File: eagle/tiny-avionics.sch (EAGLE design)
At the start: 62 parts, among them J1 USB-MICROB, J3 JST-PH-2-SMT-RA, U1 LP5907, U2 M25PX16, U3 LSM6DS3, U4 BQ21040, U5 LTC1998, U6 ATMEGA32U4-AU, X1 8MHz

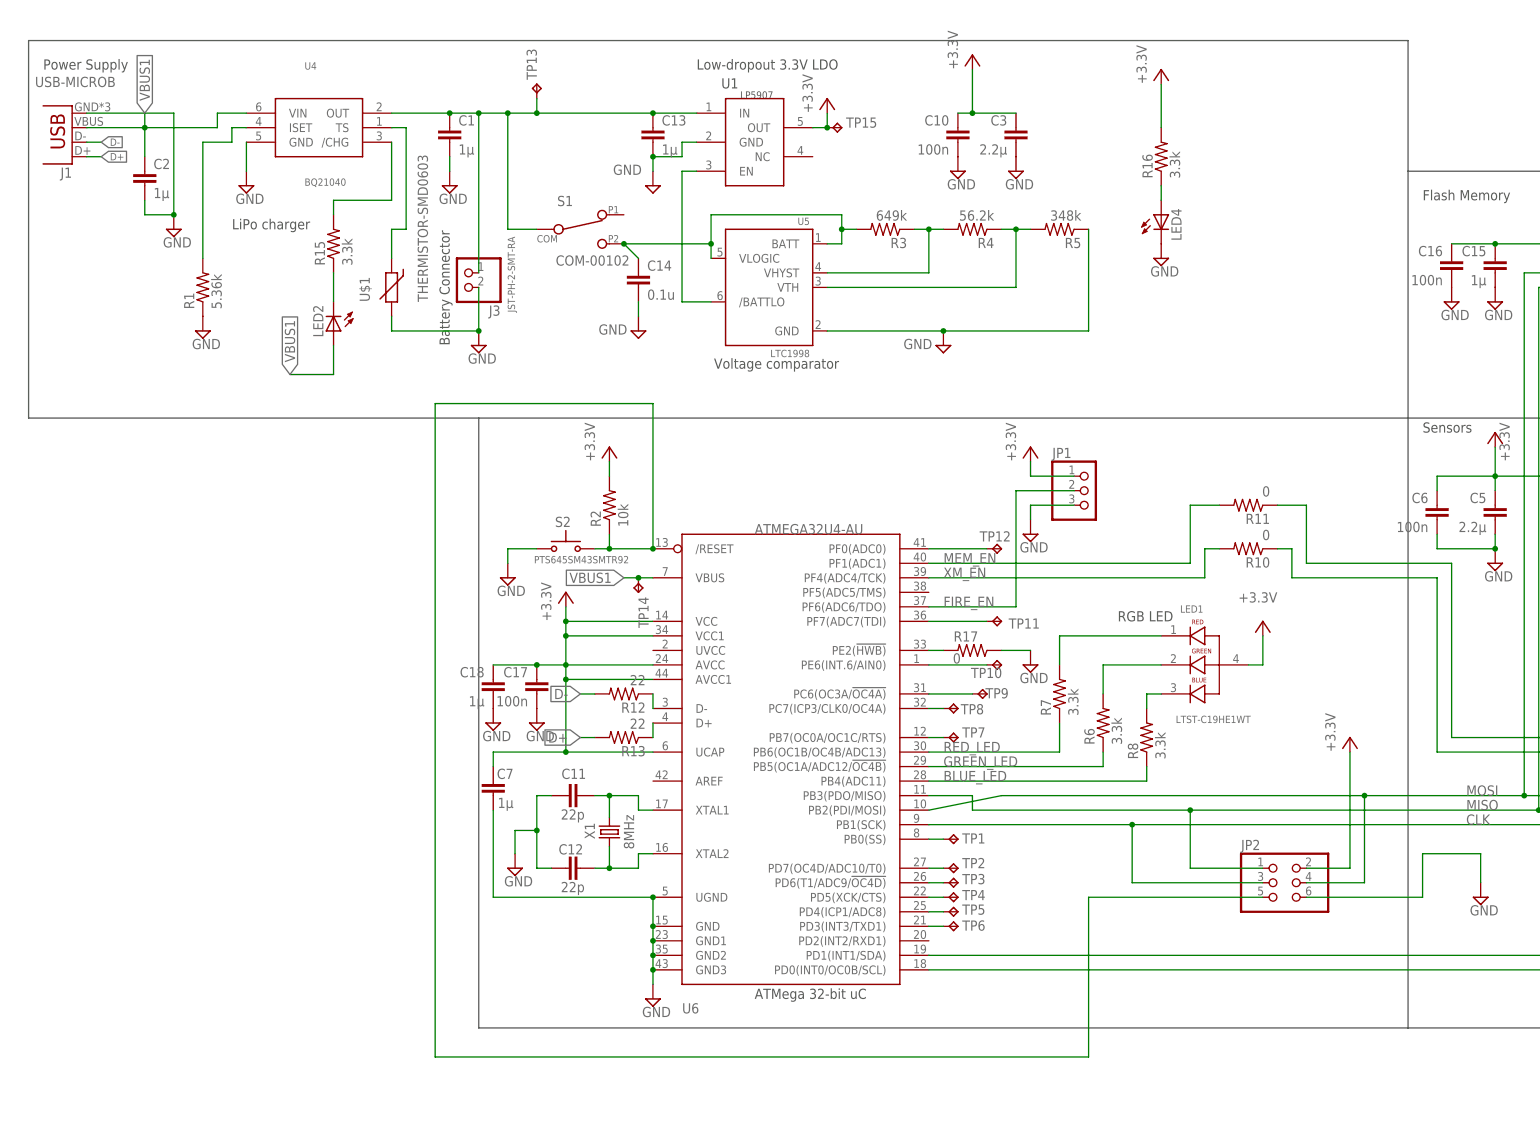
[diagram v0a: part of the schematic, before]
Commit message: Went through a few of the issues Andrew raised.  Still some that need to be addressed.
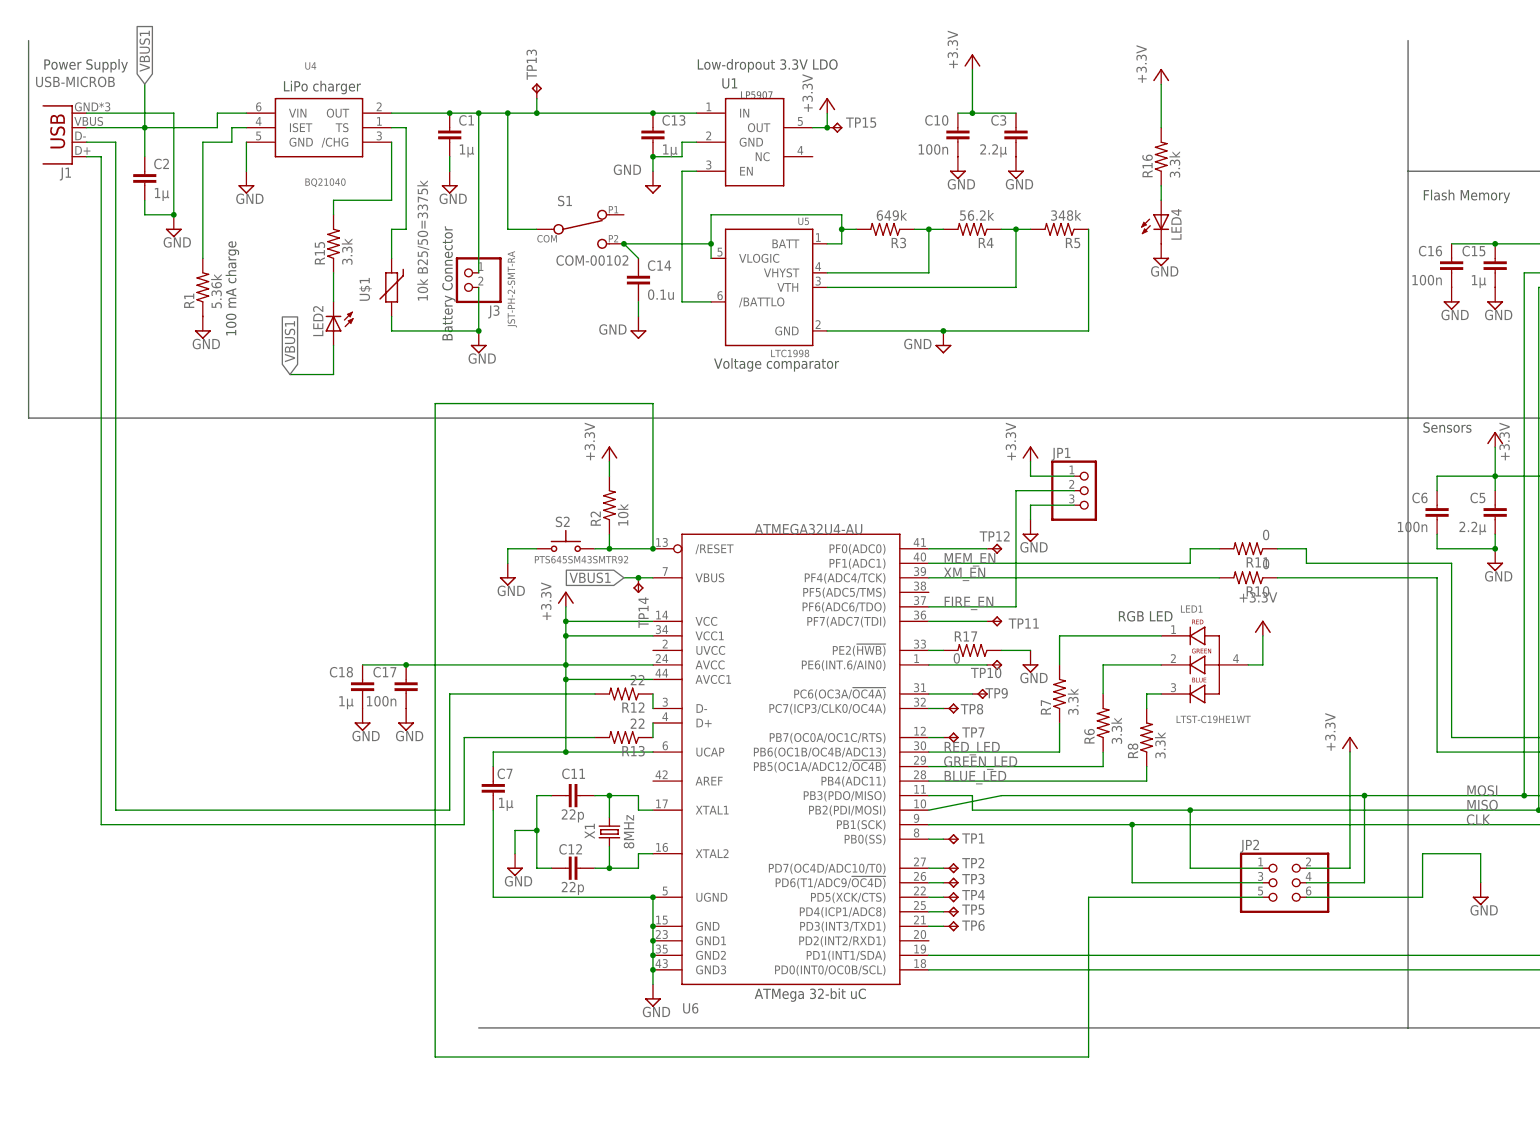
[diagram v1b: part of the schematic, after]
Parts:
- U$1: value THERMISTOR-SMD0603 -> 10k B25/50=3375k
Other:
- note added: "100 mA charge"
- moved on the sheet: C17, C18, R10, R11
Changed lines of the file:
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@@
 <part name="C3" library="rcl" deviceset="C-EU" device="C0603" value="2.2µ"/>
 <part name="SUPPLY14" library="supply2" deviceset="GND" device=""/>
-<part name="U$1" library="tinyav-lib" deviceset="THERMISTOR-SMD" device="0603"/>
+<part name="U$1" library="tinyav-lib" deviceset="THERMISTOR-SMD" device="0603" value="10k B25/50=3375k"/>
 </parts>
 <sheets>
@@
 <text x="330.2" y="25.4" size="2.54" layer="97">Model Rocket Avionics, Team 8
 Schematic Diagram</text>
-<wire x1="259.08" y1="264.16" x2="17.78" y2="264.16" width="0.1524" layer="97"/>
 <text x="20.32" y="259.08" size="1.778" layer="97">Power Supply</text>
 <wire x1="259.08" y1="91.44" x2="259.08" y2="198.12" width="0.1524" layer="97"/>
@@
 <text x="411.48" y="45.72" size="2.54" layer="97" rot="R180">All capacitors 16 V rating, ceramic
 All resistors 1%, high values 1/10W, low values 1/2 W</text>
-<text x="91.44" y="210.82" size="1.778" layer="97" rot="R90">Battery Connector</text>
+<text x="90.17" y="231.648" size="1.778" layer="97" rot="R270">Battery Connector</text>
 <wire x1="17.78" y1="264.16" x2="17.78" y2="198.12" width="0.1524" layer="97"/>
-<wire x1="17.78" y1="198.12" x2="96.52" y2="198.12" width="0.1524" layer="97"/>
 <wire x1="259.08" y1="241.3" x2="259.08" y2="264.16" width="0.1524" layer="97"/>
 <wire x1="259.08" y1="91.44" x2="96.52" y2="91.44" width="0.1524" layer="97"/>
-<wire x1="96.52" y1="91.44" x2="96.52" y2="198.12" width="0.1524" layer="97"/>
-<wire x1="96.52" y1="198.12" x2="259.08" y2="198.12" width="0.1524" layer="97"/>
+<wire x1="17.78" y1="198.12" x2="259.08" y2="198.12" width="0.1524" layer="97"/>
 <text x="134.62" y="259.08" size="1.778" layer="97">Low-dropout 3.3V LDO</text>
 <text x="137.668" y="206.756" size="1.778" layer="97">Voltage comparator</text>
-<text x="53.34" y="231.14" size="1.778" layer="97">LiPo charger</text>
+<text x="62.23" y="255.27" size="1.778" layer="97">LiPo charger</text>
 <text x="144.78" y="96.52" size="1.778" layer="97">ATMega 32-bit uC</text>
 <text x="304.292" y="238.76" size="1.778" layer="97">16Meg Flash Memory</text>
@@
 <text x="302.26" y="231.902" size="1.778" layer="97">U2</text>
 <text x="138.938" y="255.778" size="1.778" layer="97">U1</text>
+<text x="54.102" y="212.344" size="1.778" layer="97" rot="R90">100 mA charge</text>
 </plain>
 <instances>
@@
 <instance part="J3" gate="G$1" x="93.98" y="223.52" smashed="yes" rot="R180">
 <attribute name="NAME" x="100.33" y="217.805" size="1.778" layer="95" rot="R180"/>
-<attribute name="VALUE" x="101.6" y="229.87" size="1.27" layer="96" rot="R270"/>
+<attribute name="VALUE" x="101.6" y="227.33" size="1.27" layer="96" rot="R270"/>
 </instance>
 <instance part="SUPPLY2" gate="GND" x="96.52" y="210.82"/>
@@
 <instance part="SUPPLY6" gate="GND" x="266.7" y="218.44"/>
 <instance part="SUPPLY20" gate="GND" x="274.32" y="218.44"/>
-<instance part="C17" gate="G$1" x="106.68" y="152.4" rot="MR0"/>
-<instance part="C18" gate="G$1" x="99.06" y="152.4" rot="MR0"/>
-<instance part="SUPPLY21" gate="GND" x="106.68" y="144.78"/>
-<instance part="SUPPLY22" gate="GND" x="99.06" y="144.78"/>
+<instance part="C17" gate="G$1" x="83.82" y="152.4" rot="MR0"/>
+<instance part="C18" gate="G$1" x="76.2" y="152.4" rot="MR0"/>
+<instance part="SUPPLY21" gate="GND" x="83.82" y="144.78"/>
+<instance part="SUPPLY22" gate="GND" x="76.2" y="144.78"/>
 <instance part="LED1" gate="G$1" x="220.98" y="154.94">
 <attribute name="VENDOR" x="220.98" y="154.94" size="1.778" layer="96" display="off"/>
@@
 <instance part="R7" gate="G$1" x="198.12" y="149.86" rot="R90"/>
 <instance part="R8" gate="G$1" x="213.36" y="142.24" rot="R90"/>
-<instance part="R10" gate="G$1" x="231.14" y="175.26" rot="R180"/>
-<instance part="R11" gate="G$1" x="231.14" y="182.88" rot="R180"/>
+<instance part="R10" gate="G$1" x="231.14" y="170.18" rot="R180"/>
+<instance part="R11" gate="G$1" x="231.14" y="175.26" rot="R180"/>
 <instance part="R2" gate="G$1" x="119.38" y="182.88" rot="R90"/>
 <instance part="JP1" gate="A" x="203.2" y="185.42"/>
@@
 <label x="177.8" y="172.72" size="1.778" layer="95"/>
 <pinref part="R11" gate="G$1" pin="1"/>
-<wire x1="236.22" y1="182.88" x2="241.3" y2="182.88" width="0.1524" layer="91"/>
-<wire x1="241.3" y1="182.88" x2="241.3" y2="172.72" width="0.1524" layer="91"/>
+<wire x1="236.22" y1="175.26" x2="241.3" y2="175.26" width="0.1524" layer="91"/>
+<wire x1="241.3" y1="175.26" x2="241.3" y2="172.72" width="0.1524" layer="91"/>
 <wire x1="241.3" y1="172.72" x2="266.7" y2="172.72" width="0.1524" layer="91"/>
 <pinref part="U2" gate="G$1" pin="/S"/>
@@
 <label x="177.8" y="170.18" size="1.778" layer="95"/>
 <pinref part="R10" gate="G$1" pin="1"/>
-<wire x1="236.22" y1="175.26" x2="238.76" y2="175.26" width="0.1524" layer="91"/>
-<wire x1="238.76" y1="175.26" x2="238.76" y2="170.18" width="0.1524" layer="91"/>
-<wire x1="238.76" y1="170.18" x2="264.16" y2="170.18" width="0.1524" layer="91"/>
+<wire x1="236.22" y1="170.18" x2="264.16" y2="170.18" width="0.1524" layer="91"/>
 <pinref part="U3" gate="G$1" pin="CS"/>
 <wire x1="342.9" y1="180.34" x2="327.66" y2="180.34" width="0.1524" layer="91"/>
@@
 <pinref part="C18" gate="G$1" pin="1"/>
 <pinref part="C17" gate="G$1" pin="1"/>
-<wire x1="99.06" y1="154.94" x2="106.68" y2="154.94" width="0.1524" layer="91"/>
-<wire x1="106.68" y1="154.94" x2="111.76" y2="154.94" width="0.1524" layer="91"/>
-<junction x="106.68" y="154.94"/>
+<wire x1="76.2" y1="154.94" x2="83.82" y2="154.94" width="0.1524" layer="91"/>
+<wire x1="83.82" y1="154.94" x2="111.76" y2="154.94" width="0.1524" layer="91"/>
+<junction x="83.82" y="154.94"/>
 </segment>
 <segment>
@@
 <net name="D-" class="0">
 <segment>
-<wire x1="27.94" y1="246.38" x2="30.48" y2="246.38" width="0.1524" layer="91"/>
-<label x="30.48" y="246.38" size="1.27" layer="95" xref="yes"/>
+<pinref part="R12" gate="G$1" pin="2"/>
 <pinref part="J1" gate="G$1" pin="D-"/>
-</segment>
-<segment>
-<pinref part="R12" gate="G$1" pin="2"/>
-<wire x1="116.84" y1="149.86" x2="114.3" y2="149.86" width="0.1524" layer="91"/>
-<label x="114.3" y="149.86" size="1.778" layer="95" rot="R180" xref="yes"/>
+<wire x1="27.94" y1="246.38" x2="33.02" y2="246.38" width="0.1524" layer="91"/>
+<wire x1="33.02" y1="246.38" x2="33.02" y2="129.54" width="0.1524" layer="91"/>
+<wire x1="33.02" y1="129.54" x2="91.44" y2="129.54" width="0.1524" layer="91"/>
+<wire x1="91.44" y1="129.54" x2="91.44" y2="149.86" width="0.1524" layer="91"/>
+<wire x1="91.44" y1="149.86" x2="116.84" y2="149.86" width="0.1524" layer="91"/>
 </segment>
 </net>
 <net name="D+" class="0">
 <segment>
-<wire x1="27.94" y1="243.84" x2="30.48" y2="243.84" width="0.1524" layer="91"/>
-<label x="30.48" y="243.84" size="1.27" layer="95" xref="yes"/>
+<pinref part="R13" gate="G$1" pin="2"/>
+<wire x1="116.84" y1="142.24" x2="93.98" y2="142.24" width="0.1524" layer="91"/>
+<wire x1="93.98" y1="142.24" x2="93.98" y2="127" width="0.1524" layer="91"/>
+<wire x1="93.98" y1="127" x2="30.48" y2="127" width="0.1524" layer="91"/>
+<wire x1="30.48" y1="127" x2="30.48" y2="243.84" width="0.1524" layer="91"/>
 <pinref part="J1" gate="G$1" pin="D+"/>
-</segment>
-<segment>
-<pinref part="R13" gate="G$1" pin="2"/>
-<wire x1="116.84" y1="142.24" x2="114.3" y2="142.24" width="0.1524" layer="91"/>
-<label x="114.3" y="142.24" size="1.778" layer="95" rot="R180" xref="yes"/>
+<wire x1="30.48" y1="243.84" x2="27.94" y2="243.84" width="0.1524" layer="91"/>
 </segment>
 </net>
@@
 <wire x1="127" y1="170.18" x2="124.46" y2="170.18" width="0.1524" layer="91"/>
 <label x="121.92" y="170.18" size="1.778" layer="95" rot="R180" xref="yes"/>
-<label x="38.1" y="251.46" size="1.778" layer="95" rot="R90" xref="yes"/>
+<label x="38.1" y="256.54" size="1.778" layer="95" rot="R90" xref="yes"/>
 <label x="63.5" y="205.74" size="1.778" layer="95" rot="R90" xref="yes"/>
 <pinref part="TP14" gate="G$1" pin="TP"/>
@@
 <wire x1="27.94" y1="248.92" x2="38.1" y2="248.92" width="0.1524" layer="91"/>
 <junction x="38.1" y="248.92"/>
-<wire x1="38.1" y1="248.92" x2="38.1" y2="251.46" width="0.1524" layer="91"/>
 <wire x1="38.1" y1="248.92" x2="50.8" y2="248.92" width="0.1524" layer="91"/>
 <wire x1="50.8" y1="248.92" x2="50.8" y2="251.46" width="0.1524" layer="91"/>
 <pinref part="U4" gate="BQ21040" pin="VIN"/>
 <wire x1="50.8" y1="251.46" x2="55.88" y2="251.46" width="0.1524" layer="91"/>
+<wire x1="38.1" y1="248.92" x2="38.1" y2="256.54" width="0.1524" layer="91"/>
 </segment>
 <segment>
@@
 <segment>
 <pinref part="U6" gate="G$1" pin="PF4(ADC4/TCK)"/>
-<wire x1="175.26" y1="170.18" x2="223.52" y2="170.18" width="0.1524" layer="91"/>
-<wire x1="223.52" y1="170.18" x2="223.52" y2="175.26" width="0.1524" layer="91"/>
+<wire x1="175.26" y1="170.18" x2="226.06" y2="170.18" width="0.1524" layer="91"/>
 <pinref part="R10" gate="G$1" pin="2"/>
-<wire x1="223.52" y1="175.26" x2="226.06" y2="175.26" width="0.1524" layer="91"/>
 </segment>
 </net>
@@
 <pinref part="U6" gate="G$1" pin="PF1(ADC1)"/>
 <wire x1="175.26" y1="172.72" x2="220.98" y2="172.72" width="0.1524" layer="91"/>
-<wire x1="220.98" y1="172.72" x2="220.98" y2="182.88" width="0.1524" layer="91"/>
+<wire x1="220.98" y1="172.72" x2="220.98" y2="175.26" width="0.1524" layer="91"/>
 <pinref part="R11" gate="G$1" pin="2"/>
-<wire x1="220.98" y1="182.88" x2="226.06" y2="182.88" width="0.1524" layer="91"/>
-</segment>
-</net>
+<wire x1="220.98" y1="175.26" x2="226.06" y2="175.26" width="0.1524" layer="91"/>
+</segment>
+</net>
